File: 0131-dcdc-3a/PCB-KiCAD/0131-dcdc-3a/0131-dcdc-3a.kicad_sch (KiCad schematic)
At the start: 12 parts, among them U1 AP62300WU

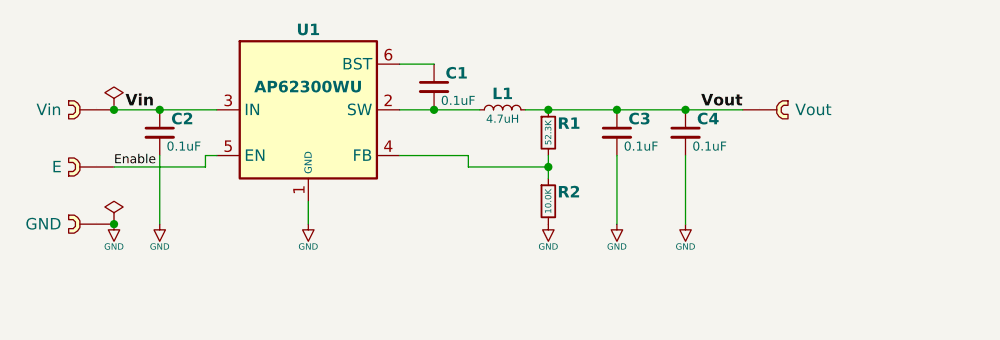
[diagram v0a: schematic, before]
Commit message: Tune documentation, info block.
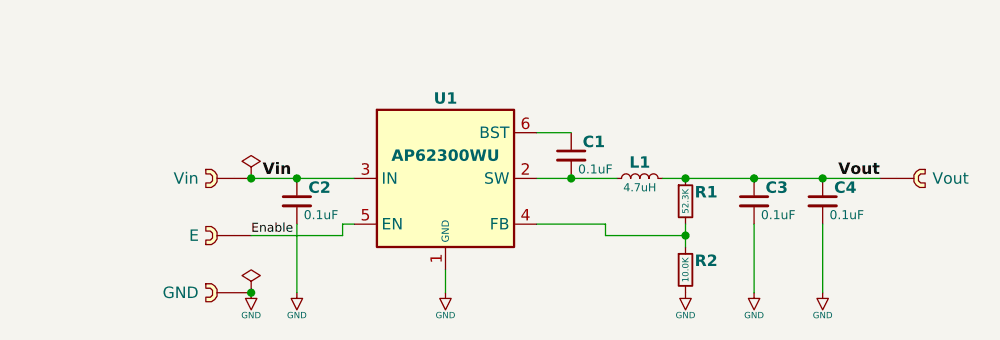
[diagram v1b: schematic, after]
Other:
- company: (none) -> Circuit Monkey
- title: (none) -> #0131 DC-DC Converter, 3A
- moved on the sheet: C1, C2, C3, C4, L1, R1, R2, U1
